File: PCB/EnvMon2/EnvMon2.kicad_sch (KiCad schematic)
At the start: 40 parts, among them J1 USB-C, J2 DC, J3 TEMP, J4 Shelly, M1 OLED1.5-RGB, SW1 SW_Push, SW2 SW_Push, SW3 SW_Push, U1 LMR16006XDDCR, U2 SCD41, U3 FT231XQ, U4 ESP32-PICO-MINI-02, U5 QR, U6 VEML3235SL_RA, U7 SHT40

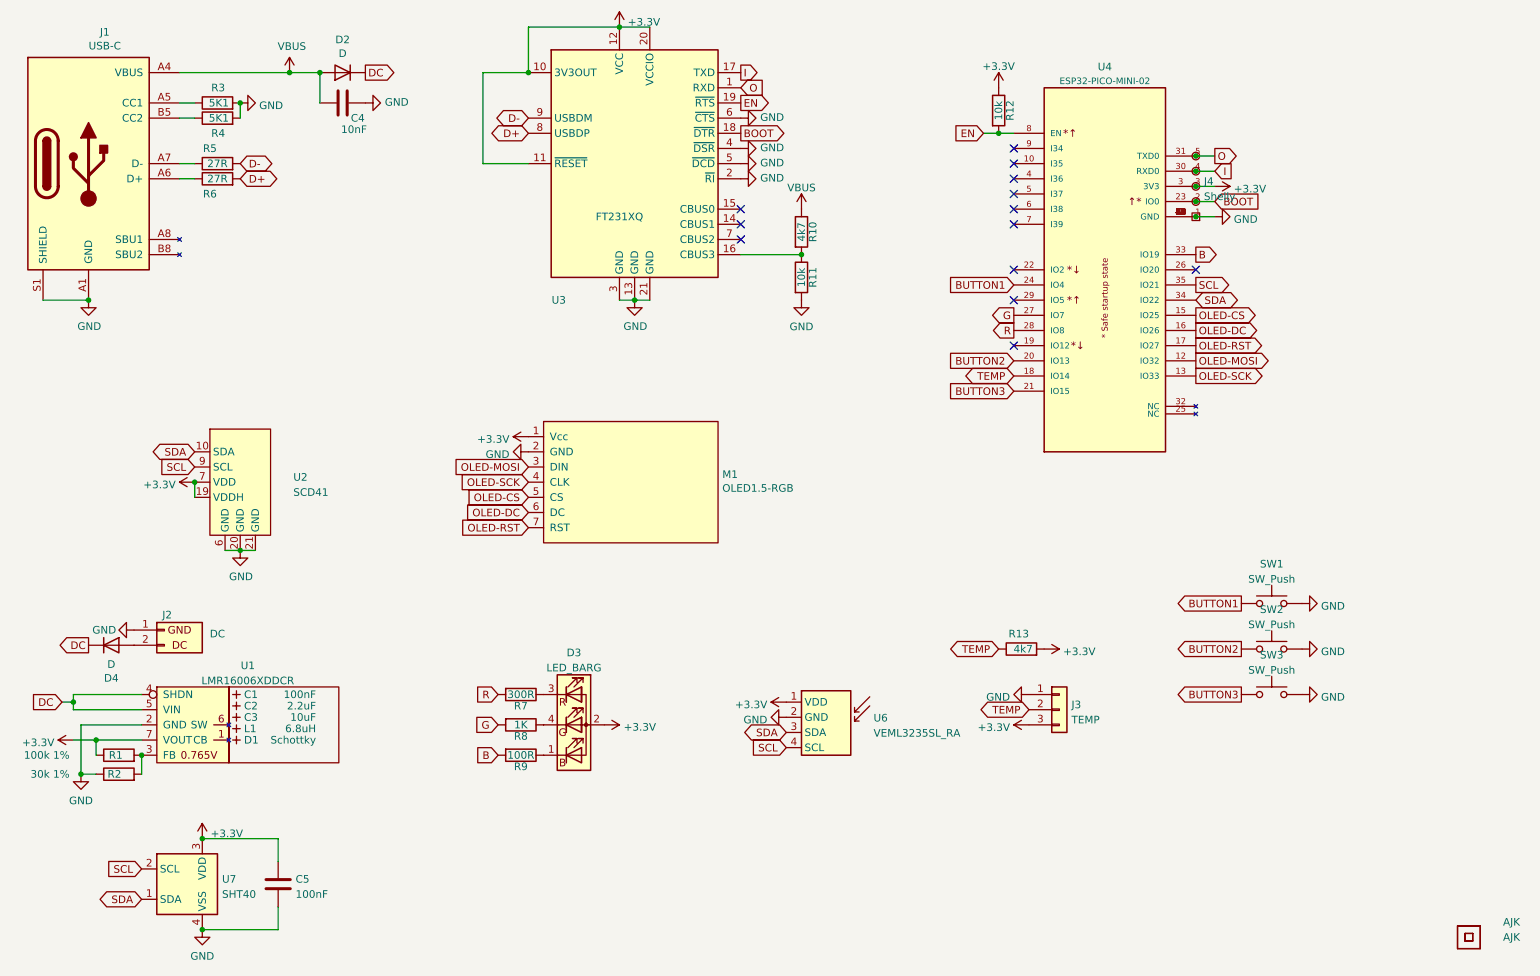
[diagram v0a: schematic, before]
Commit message: Silk and change VEML
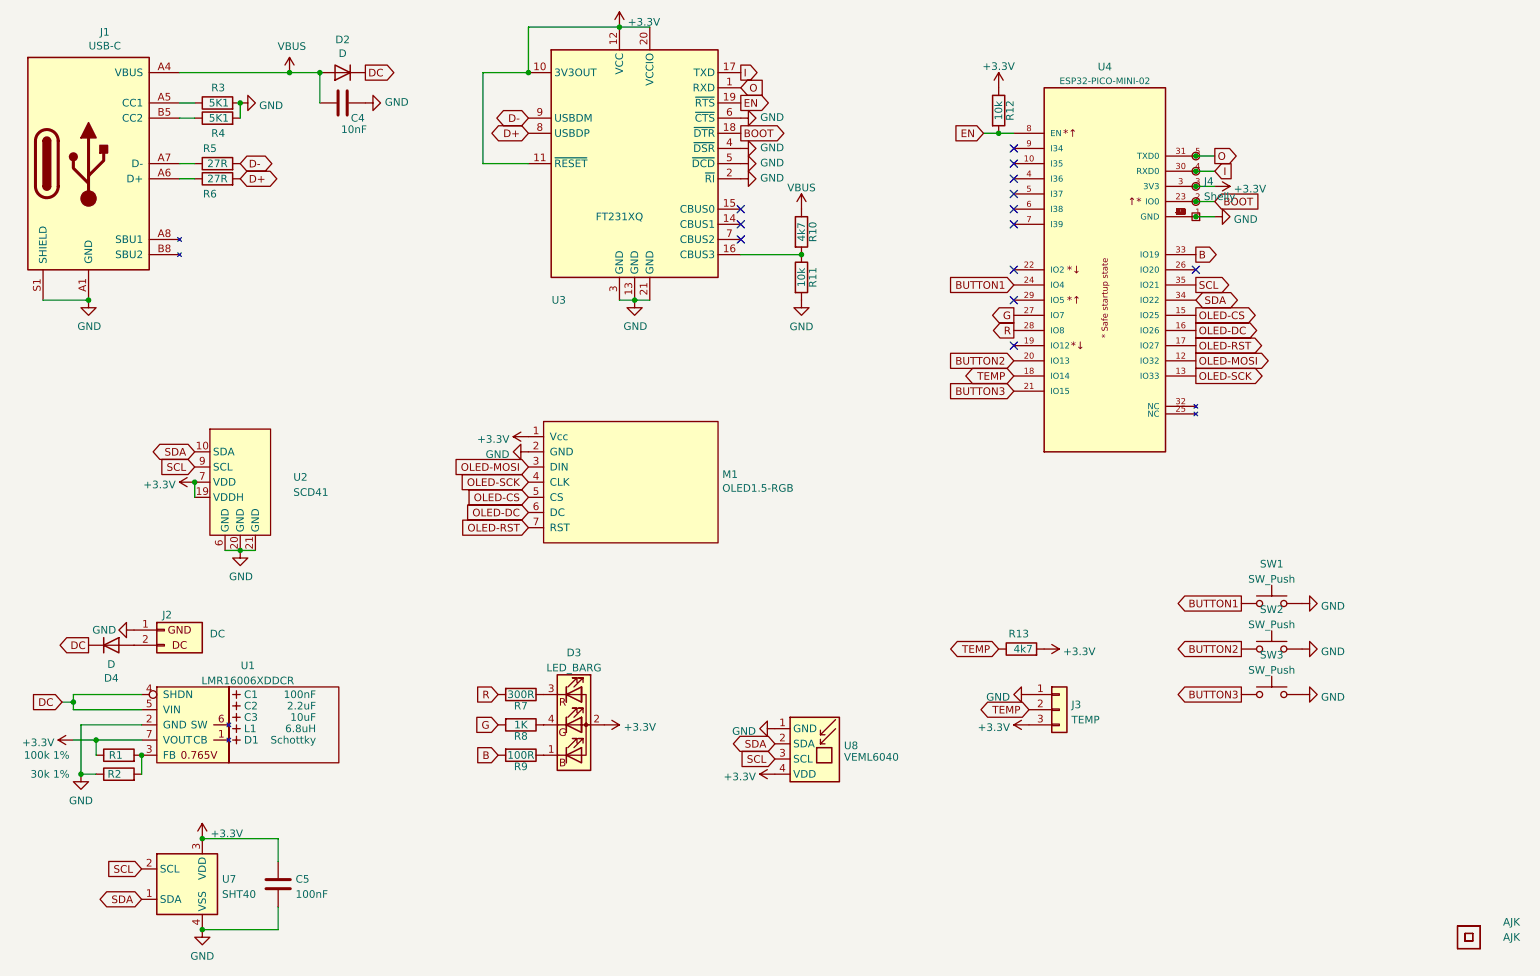
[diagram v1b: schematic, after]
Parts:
- removed U6: VEML3235SL_RA, RevK:VEML3235SL-RA, symbol RevK:VEML3235SL_RA
- added U8: VEML6040, RevK:VEML6040, symbol RevK:VEML6040
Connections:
- net +3.3V: now also U8.4 (VDD)
- net GND: now also U8.1 (GND)
- net SCL: now also U8.3 (SCL)
- net SDA: now also U8.2 (SDA)
